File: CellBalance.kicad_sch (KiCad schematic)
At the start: 9 parts

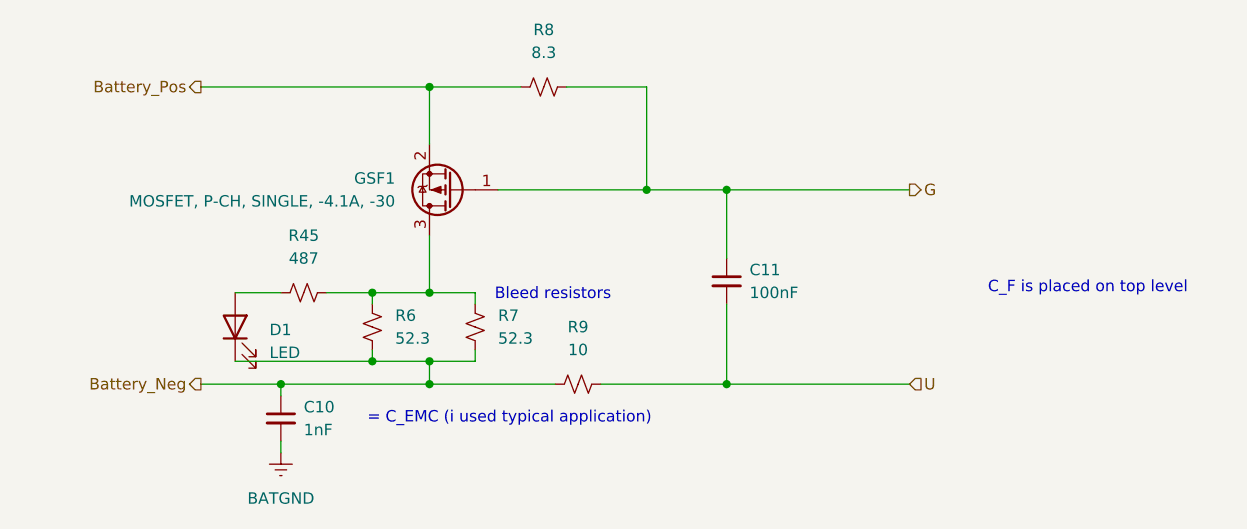
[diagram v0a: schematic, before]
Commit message: passive values
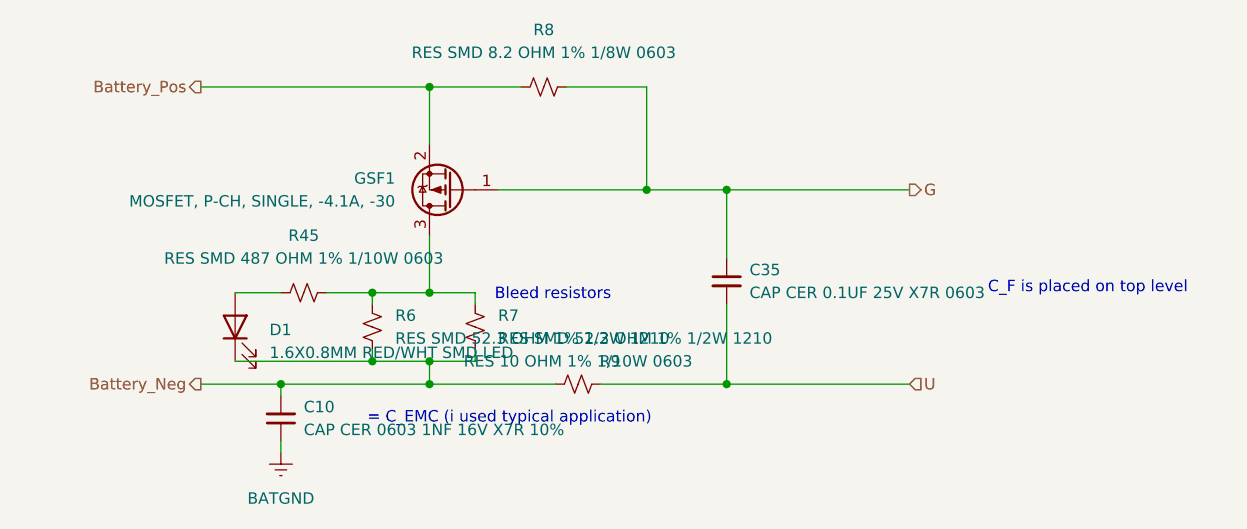
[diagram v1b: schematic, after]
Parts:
- removed C11: 100nF, symbol Device:C_Small
- added C35: CAP CER 0.1UF 25V X7R 0603, Capacitor_SMD:C_0603_1608Metric, symbol Device:C_Small
- C10: value 1nF -> CAP CER 0603 1NF 16V X7R 10%; footprint (none) -> Capacitor_SMD:C_0603_1608Metric
- D1: value LED -> 1.6X0.8MM RED/WHT SMD LED; footprint (none) -> Diode_SMD:D_0603_1608Metric
- R45: value 487 -> RES SMD 487 OHM 1% 1/10W 0603; footprint (none) -> Capacitor_SMD:C_0603_1608Metric
- R6, R7: value 52.3 -> RES SMD 52.3 OHM 1% 1/2W 1210; footprint (none) -> Capacitor_SMD:C_1210_3225Metric
- R8: value 8.3 -> RES SMD 8.2 OHM 1% 1/8W 0603; footprint (none) -> Capacitor_SMD:C_0603_1608Metric
- R9: value 10 -> RES 10 OHM 1% 1/10W 0603; footprint (none) -> Resistor_SMD:R_0603_1608Metric
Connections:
- net BATGND: now also C10.1; no longer C10.2
- net Battery_Neg: now also C10.2; no longer C10.1
- net G: now also C35.1
- net U: now also C35.2
